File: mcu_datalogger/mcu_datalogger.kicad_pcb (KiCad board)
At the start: 2 copper layers, 51.9 x 31.1 mm, 29 parts, among them J1 Conn_01x04_Pin, J2 Conn_01x04_Pin, J3 Conn_01x09, J4 Conn_02x03_Odd_Even, U1 24LC1025, U2 24LC1025, U3 DS1337S_, U4 ATMEGA328P-AU, Y1 16MHz, Y2 32.768 KHz

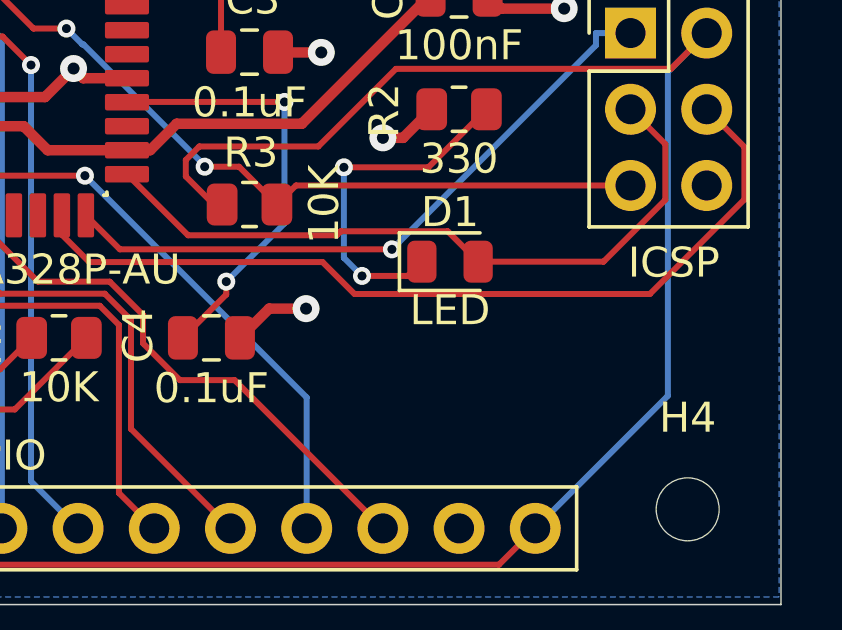
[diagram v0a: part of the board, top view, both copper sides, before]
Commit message: add graphics to mcu
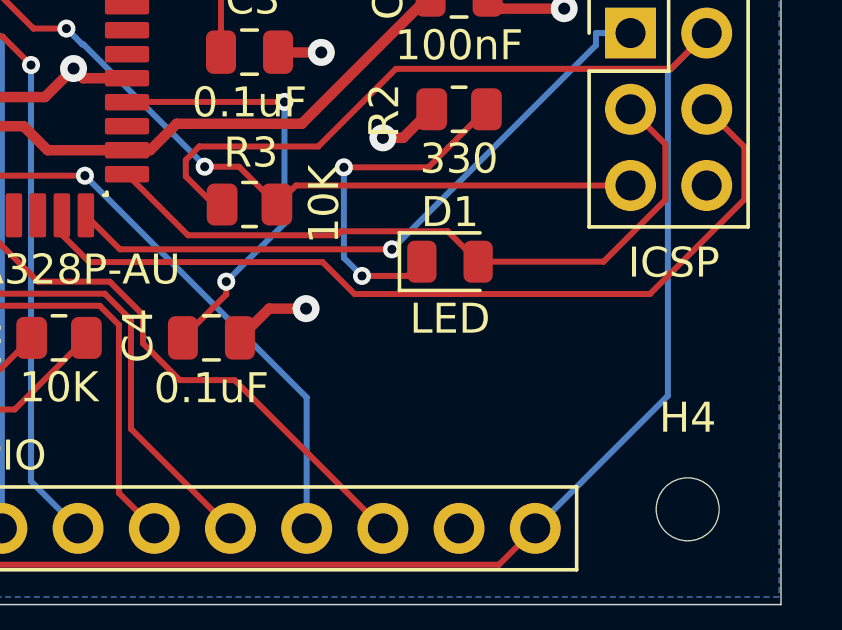
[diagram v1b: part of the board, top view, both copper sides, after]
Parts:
- added G***: LOGO, JPI_LOGOS:jpi_logo_10mm_silkscreen, B.Cu at (78.1, 56.5)
- added G***: LOGO, JPI_LOGOS:shodan_10mm_silkscreen, B.Cu at (103.5, 67.9)
